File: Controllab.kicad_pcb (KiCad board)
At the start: 2 copper layers, 56.5 x 70 mm, 57 parts, among them J3 TYPE-C-31-M-12, SW1 SW_Push, SW2 SW_Push, U2 ESP32-S3-MINI-1, U3 PN5321A3HN_C1xx, U4 AMS1117-3.3, Y1 Crystal

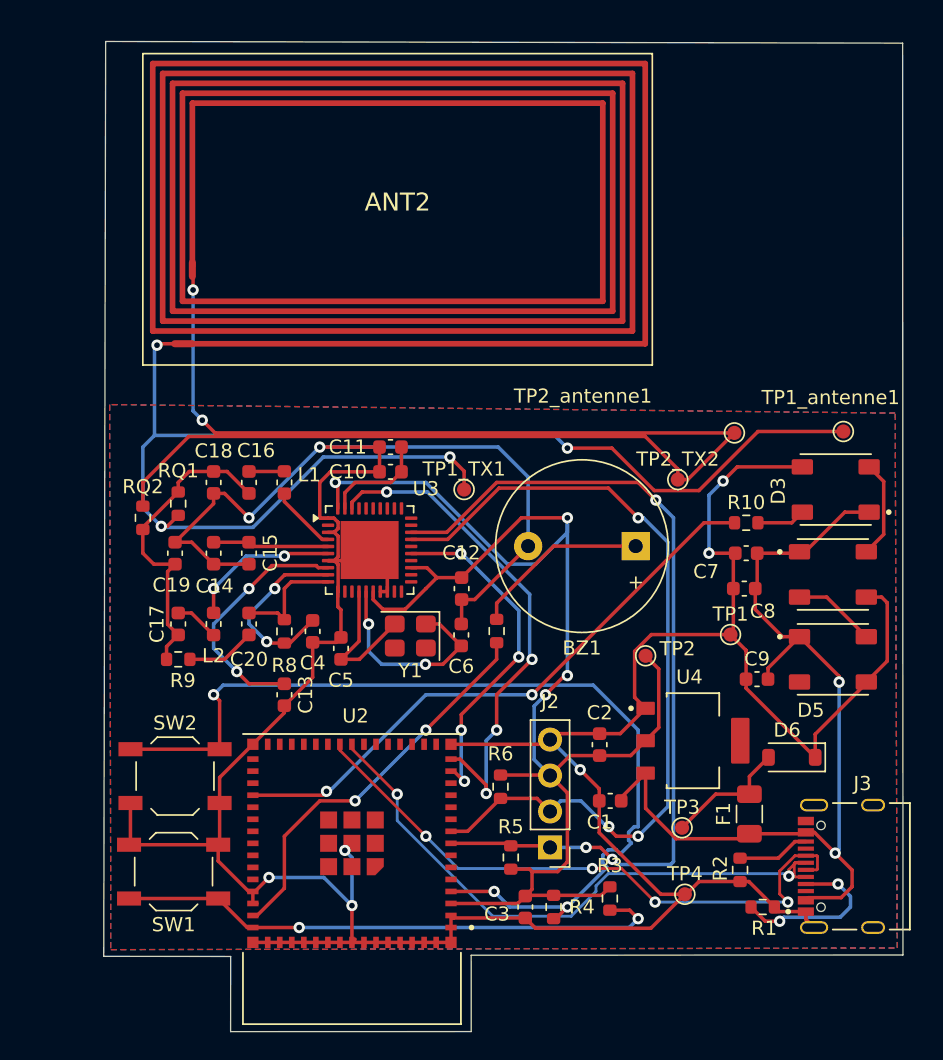
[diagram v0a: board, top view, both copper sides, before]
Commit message: La carte est prete
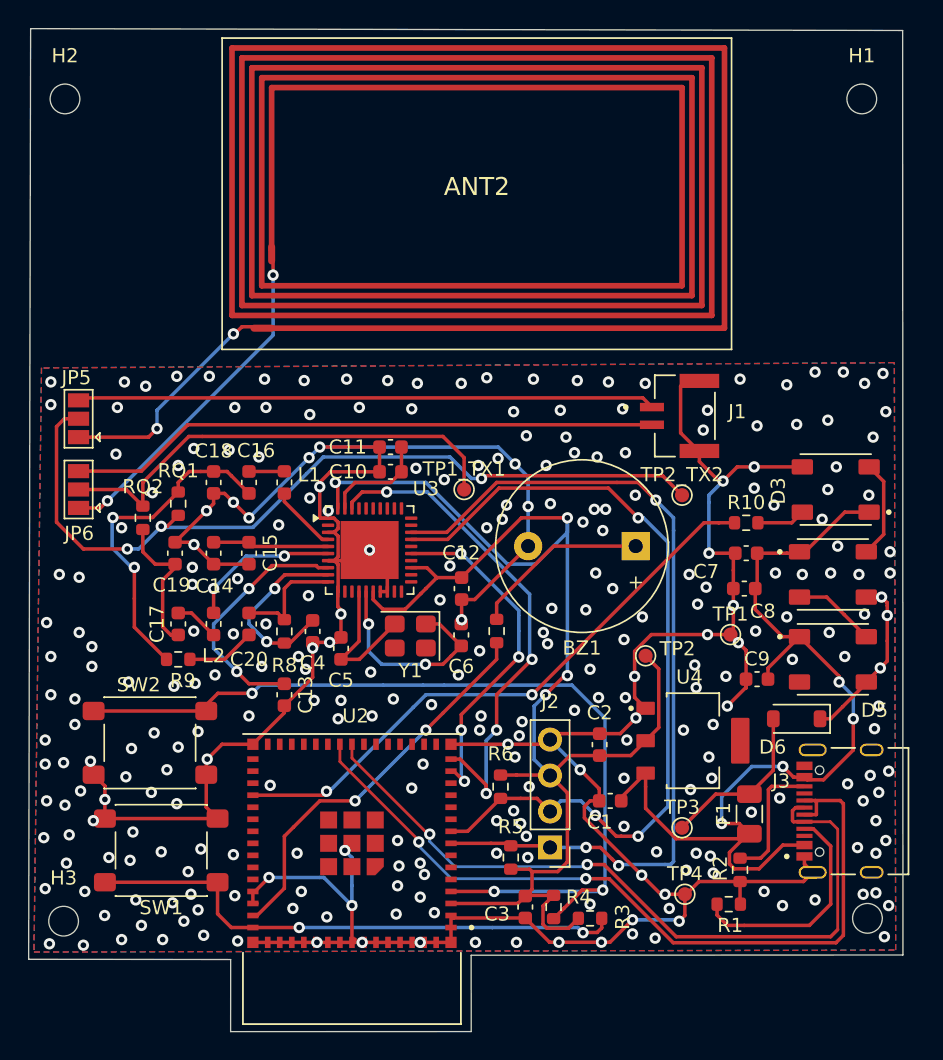
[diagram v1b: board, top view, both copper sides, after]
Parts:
- removed TP1_antenne1, TP2_antenne1: TestPoint, TestPoint:TestPoint_Pad_D1.0mm
- added H1: MountingHole, MountingHole:MountingHole_2.1mm, F.Cu at (140.8, 95.4)
- added H2: MountingHole, MountingHole:MountingHole_2.1mm, F.Cu at (84.5, 95.4)
- added H3: MountingHole, MountingHole:MountingHole_2.1mm, F.Cu at (84.4, 153.5)
- added H4: MountingHole, MountingHole:MountingHole_2.1mm, F.Cu at (141.2, 153.3)
- added J1: BM02B-GHS-TBT_LF__SN__N_, connecteur_pretty:JST_BM02B-GHS-TBT_LF__SN__N_, F.Cu at (128.3, 117.8)
- added JP5: SolderJumper_3_Open, Jumper:SolderJumper-3_P1.3mm_Open_Pad1.0x1.5mm, F.Cu at (85.5, 118.0)
- added JP6: SolderJumper_3_Open, Jumper:SolderJumper-3_P1.3mm_Open_Pad1.0x1.5mm, F.Cu at (85.5, 123.0)
- R9: value 22K -> 2.7K
- SW1, SW2: footprint Button_Switch_SMD:SW_SPST_TL3342 -> Button_Switch_SMD:SW_SPST_PTS645Sx43SMTR92
- moved ANT2 5.71 mm to (113.6, 101.6)
- moved J3 3.90 mm to (141.5, 145.7)
- moved SW2 2.95 mm to (90.5, 140.9)
- moved D6 2.75 mm to (136.2, 139.2)
- moved R1 2.41 mm to (131.4, 152.3)
- moved R3 1.98 mm to (121.6, 153.3), turned to 0 degrees
- moved SW1 1.74 mm to (91.3, 148.5)
- moved TP2_TX2 1.14 mm to (128.1, 123.4)
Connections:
- C17 pad 2: Net-(C16-Pad2) -> Net-(C17-Pad2)
- C19 pad 1: Net-(C16-Pad2) -> Net-(C17-Pad2)
- RQ1 pad 2: Net-(ANT2-T1) -> Net-(JP5-C)
- RQ2 pad 1: Net-(C16-Pad2) -> Net-(C17-Pad2)
- RQ2 pad 2: Net-(ANT2-T2) -> Net-(JP6-C)
- TP1_TX1 pad 1: Net-(ANT2-T1) -> Net-(JP6-C)
- TP2_TX2 pad 1: Net-(ANT2-T2) -> Net-(JP5-C)
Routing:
- net Net-(ANT2-T1): track 94.1 -> 16.8 mm, vias 4 -> 2
- net Net-(ANT2-T2): track 96.6 -> 24.4 mm
- net Net-(JP5-C): track 0.00 -> 59.1 mm, vias 0 -> 3
- net Net-(JP6-B): track 0.00 -> 41.9 mm
- net Net-(JP5-B): track 0.00 -> 40.9 mm
- net Net-(JP6-C): track 0.00 -> 33.6 mm
- net /USB_D+: track 43.8 -> 56.6 mm, vias 4 -> 2
- net Net-(C17-Pad2): track 0.00 -> 10.3 mm
- net /USB_D-: track 43.2 -> 53.4 mm
- net GND: track 264.0 -> 269.7 mm, vias 8 -> 291
- net VBUS: track 64.3 -> 68.6 mm, vias 2 -> 4
- net Net-(J3-CC1): track 12.1 -> 16.2 mm, vias 2 -> 0
- net Net-(J3-CC2): track 5.14 -> 9.17 mm
- net Net-(D6-A2): track 8.90 -> 11.8 mm
- net /GPIO0: track 68.2 -> 65.7 mm
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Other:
- board size 56.5 x 70 mm -> 61.8 x 70.9 mm
